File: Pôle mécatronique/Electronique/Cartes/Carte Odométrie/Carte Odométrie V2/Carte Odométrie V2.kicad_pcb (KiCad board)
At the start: 2 copper layers, 49.5 x 58.4 mm, 8 parts

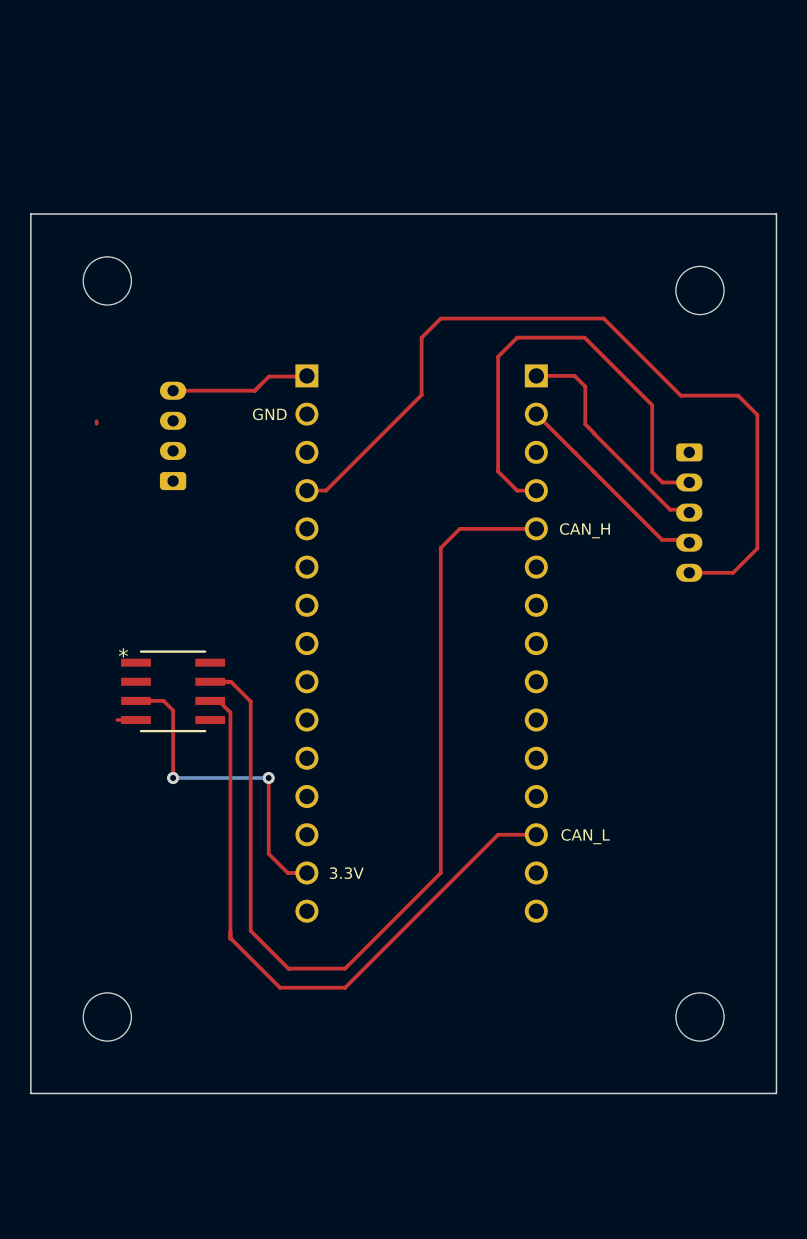
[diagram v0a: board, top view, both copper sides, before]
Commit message: Update Carte Odométrie
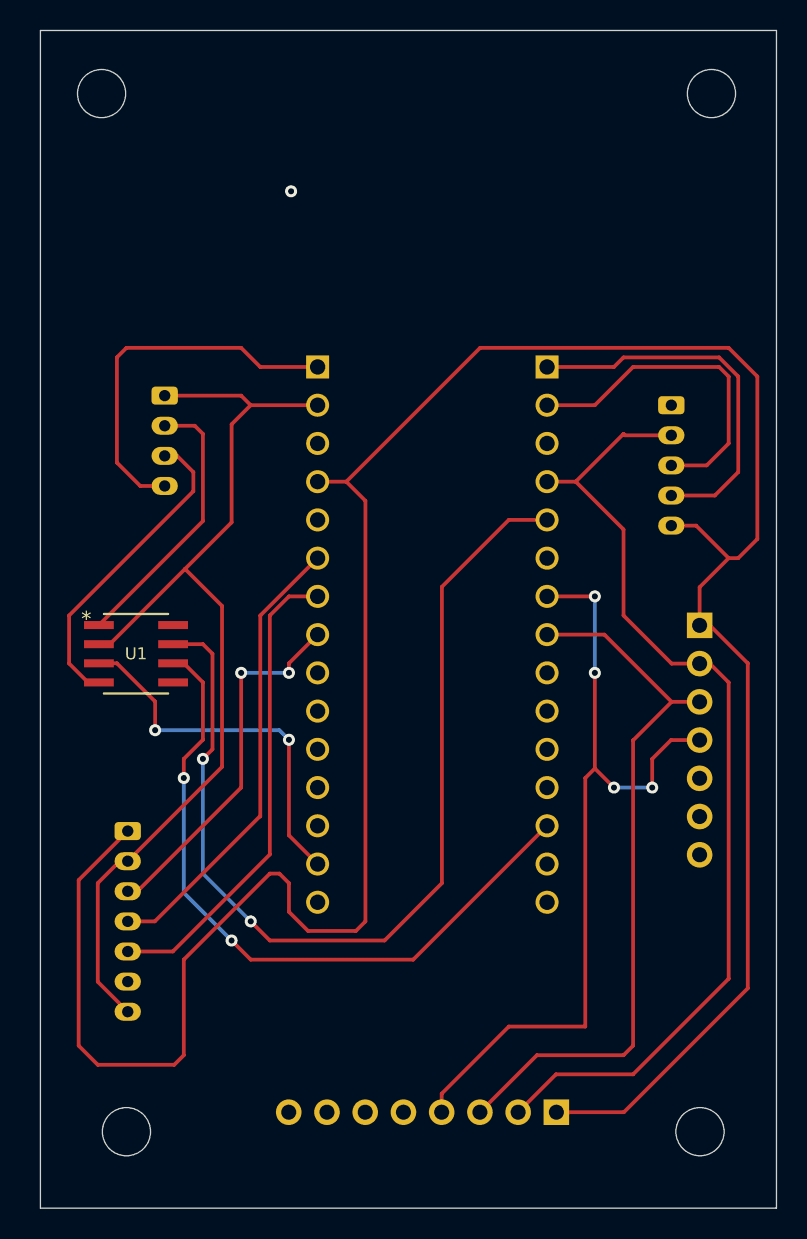
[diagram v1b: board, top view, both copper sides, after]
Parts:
- removed BUSCAN+ALIM: Conn_01x04, Connector_JST:JST_PH_B4B-PH-K_1x04_P2.00mm_Vertical
- removed CAN_Transceiver1: TCAN332, empreinte:SO-8_S
- removed Lidar: Conn_01x05, Connector_JST:JST_PH_B5B-PH-K_1x05_P2.00mm_Vertical
- removed STM32 f303k8: NUCLEO-F303K8, empreinte:MODULE_NUCLEO-F303K8
- added A1: NUCLEO-F303K8, empreinte:MODULE_NUCLEO-F303K8, B.Cu at (149.9, 101.6)
- added G***: LOGO, Logos:logoRobotechNancy10x10, B.Cu at (160.2, 70.4)
- added J1: Conn_01x08, Connector_PinSocket_2.54mm:PinSocket_1x08_P2.54mm_Vertical, B.Cu at (158.1, 133.3)
- added J2: Conn_01x05, Connector_JST:JST_PH_B5B-PH-K_1x05_P2.00mm_Vertical, B.Cu at (165.7, 86.4)
- added J3: Conn_01x04, Connector_JST:JST_PH_B4B-PH-K_1x04_P2.00mm_Vertical, B.Cu at (132.1, 85.7)
- added J4: Conn_01x07, Connector_JST:JST_PH_B7B-PH-K_1x07_P2.00mm_Vertical, B.Cu at (129.6, 114.7)
- added J5: Conn_01x07, Connector_PinSocket_2.54mm:PinSocket_1x07_P2.54mm_Vertical, B.Cu at (167.6, 101.0)
- added U1: TCAN332, empreinte:SO-8_S, F.Cu at (130.2, 102.9)
- moved REF 13.1 mm to (168.4, 65.7)
- moved REF 12.5 mm to (127.9, 65.7)
- moved REF 7.73 mm to (129.5, 134.6)
- moved REF 7.62 mm to (167.6, 134.6)
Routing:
- net +5V: track 53.7 -> 175.7 mm
- net GND: track 31.6 -> 131.9 mm
- net I2C_SDA: track 0.00 -> 54.5 mm, vias 0 -> 4
- net I2C_SCL: track 0.00 -> 47.9 mm
- net SPI_MISO: track 0.00 -> 31.7 mm
- net SPI_MOSI: track 0.00 -> 30.5 mm
- net SPI_CLK: track 0.00 -> 24.5 mm, vias 0 -> 2
- net CAN_TX: track 0.00 -> 21.0 mm
- net CAN_RX: track 1.24 -> 18.3 mm
- net +BATT: track 9.85 -> 24.9 mm
- net UART1_TX: track 15.4 -> 24.9 mm
- net UART1_RX: track 13.8 -> 22.2 mm
- net CAN_L: track 43.0 -> 46.7 mm, vias 0 -> 2
- net +3V3: track 21.6 -> 24.9 mm
- net CAN_H: track 64.4 -> 65.6 mm, vias 0 -> 2
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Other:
- board size 49.5 x 58.4 mm -> 48.9 x 78.2 mm
- board text added: "I2C_SDA"
- board text added: "I2C_SDL"
- board text added: "ROBOTECH NANCY"
- board text added: "SPI_CLK"
- board text added: "SPI_MISO"
- board text added: "SPI_MOSI"
- board text removed: "3.3V"
- board text removed: "CAN_H"
- board text removed: "CAN_L"
